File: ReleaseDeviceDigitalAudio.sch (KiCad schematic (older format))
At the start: 5 parts, among them J1 AudioJack3, J2 AudioJack3, J3 AudioJack3, J4 AudioJack3, J5 AudioJack3

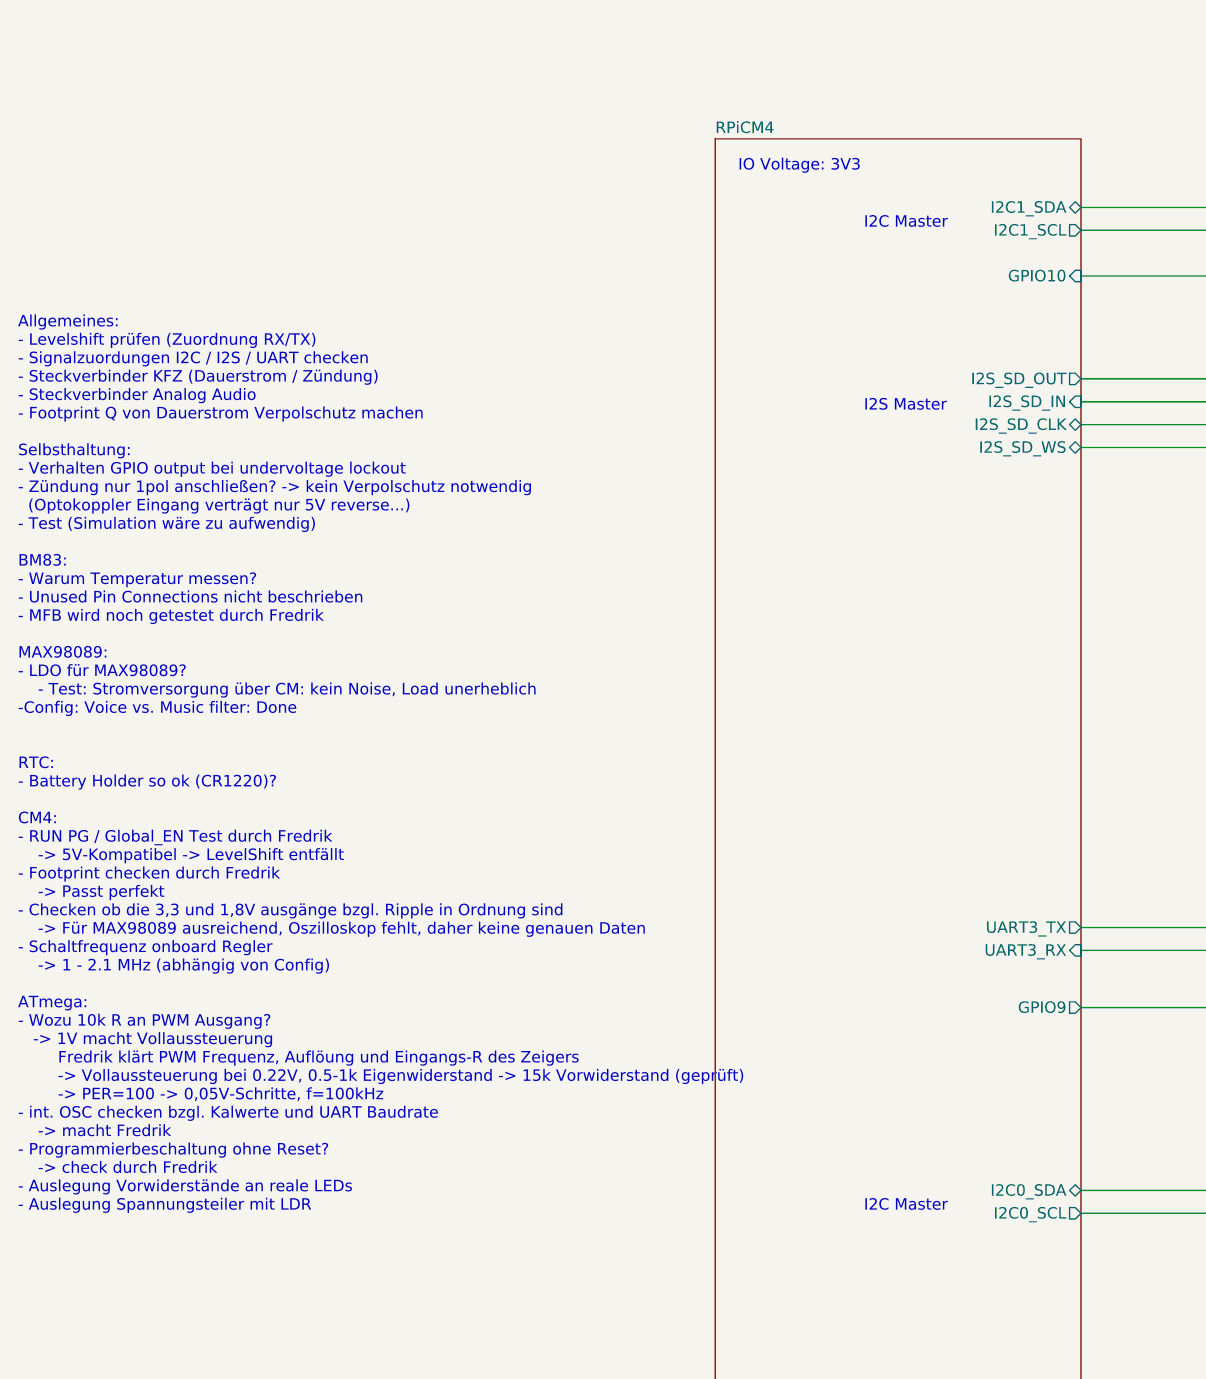
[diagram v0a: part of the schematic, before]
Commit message: - Kommentare aktualisiert
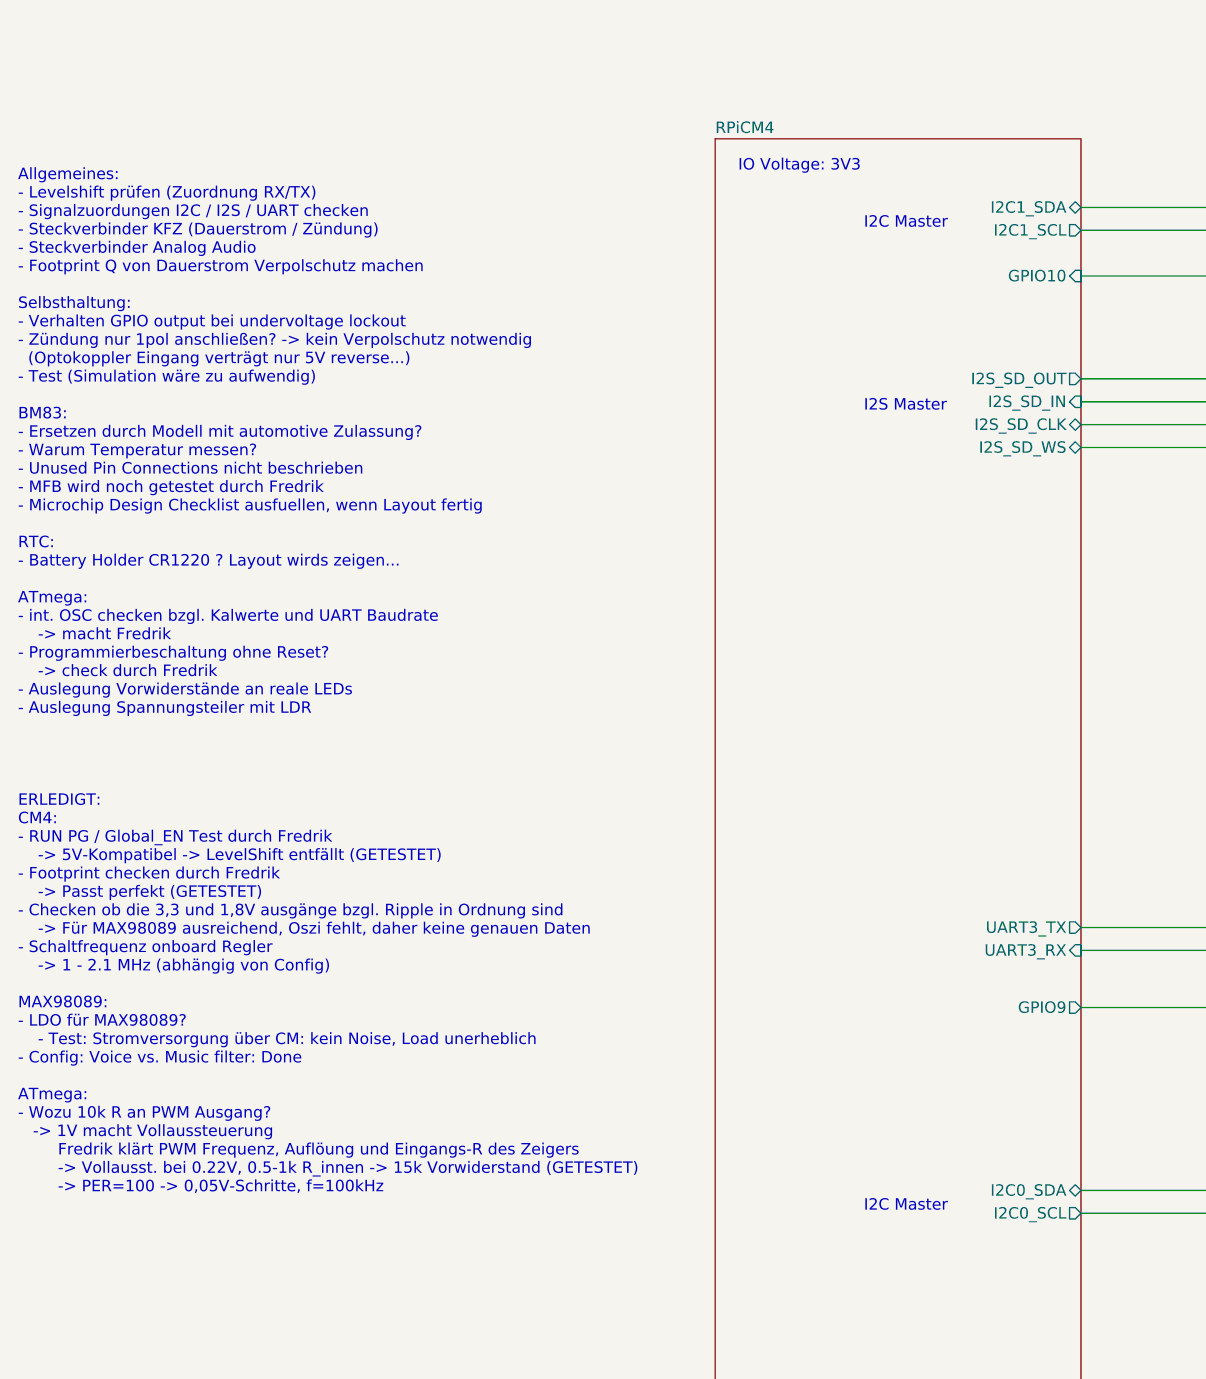
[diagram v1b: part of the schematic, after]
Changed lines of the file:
@@
 $EndComp
 Text Notes 900  5800 0    50   ~ 0
-Allgemeines: \n- Levelshift prüfen (Zuordnung RX/TX)\n- Signalzuordungen I2C / I2S / UART checken\n- Steckverbinder KFZ (Dauerstrom / Zündung)\n- Steckverbinder Analog Audio\n- Footprint Q von Dauerstrom Verpolschutz machen\n\nSelbsthaltung:\n- Verhalten GPIO output bei undervoltage lockout\n- Zündung nur 1pol anschließen? -> kein Verpolschutz notwendig\n  (Optokoppler Eingang verträgt nur 5V reverse...)\n- Test (Simulation wäre zu aufwendig)\n\nBM83:\n- Warum Temperatur messen?\n- Unused Pin Connections nicht beschrieben\n- MFB wird noch getestet durch Fredrik\n\nMAX98089:\n- LDO für MAX98089? \n    - Test: Stromversorgung über CM: kein Noise, Load unerheblich\n-Config: Voice vs. Music filter: Done\n\n\nRTC:\n- Battery Holder so ok (CR1220)?\n\nCM4: \n- RUN PG / Global_EN Test durch Fredrik\n    -> 5V-Kompatibel -> LevelShift entfällt\n- Footprint checken durch Fredrik\n    -> Passt perfekt\n- Checken ob die 3,3 und 1,8V ausgänge bzgl. Ripple in Ordnung sind\n    -> Für MAX98089 ausreichend, Oszilloskop fehlt, daher keine genauen Daten\n- Schaltfrequenz onboard Regler\n    -> 1 - 2.1 MHz (abhängig von Config)\n\nATmega:\n- Wozu 10k R an PWM Ausgang?\n   -> 1V macht Vollaussteuerung\n        Fredrik klärt PWM Frequenz, Auflöung und Eingangs-R des Zeigers\n        -> Vollaussteuerung bei 0.22V, 0.5-1k Eigenwiderstand -> 15k Vorwiderstand (geprüft)\n        -> PER=100 -> 0,05V-Schritte, f=100kHz\n- int. OSC checken bzgl. Kalwerte und UART Baudrate\n    -> macht Fredrik\n- Programmierbeschaltung ohne Reset?\n    -> check durch Fredrik\n- Auslegung Vorwiderstände an reale LEDs\n- Auslegung Spannungsteiler mit LDR\n
+Allgemeines: \n- Levelshift prüfen (Zuordnung RX/TX)\n- Signalzuordungen I2C / I2S / UART checken\n- Steckverbinder KFZ (Dauerstrom / Zündung)\n- Steckverbinder Analog Audio\n- Footprint Q von Dauerstrom Verpolschutz machen\n\nSelbsthaltung:\n- Verhalten GPIO output bei undervoltage lockout\n- Zündung nur 1pol anschließen? -> kein Verpolschutz notwendig\n  (Optokoppler Eingang verträgt nur 5V reverse...)\n- Test (Simulation wäre zu aufwendig)\n\nBM83:\n- Ersetzen durch Modell mit automotive Zulassung?\n- Warum Temperatur messen?\n- Unused Pin Connections nicht beschrieben\n- MFB wird noch getestet durch Fredrik\n- Microchip Design Checklist ausfuellen, wenn Layout fertig\n\nRTC:\n- Battery Holder CR1220 ? Layout wirds zeigen...\n\nATmega:\n- int. OSC checken bzgl. Kalwerte und UART Baudrate\n    -> macht Fredrik\n- Programmierbeschaltung ohne Reset?\n    -> check durch Fredrik\n- Auslegung Vorwiderstände an reale LEDs\n- Auslegung Spannungsteiler mit LDR\n\n\n\n\nERLEDIGT:\nCM4: \n- RUN PG / Global_EN Test durch Fredrik\n    -> 5V-Kompatibel -> LevelShift entfällt (GETESTET)\n- Footprint checken durch Fredrik\n    -> Passt perfekt (GETESTET)\n- Checken ob die 3,3 und 1,8V ausgänge bzgl. Ripple in Ordnung sind\n    -> Für MAX98089 ausreichend, Oszi fehlt, daher keine genauen Daten\n- Schaltfrequenz onboard Regler\n    -> 1 - 2.1 MHz (abhängig von Config)\n\nMAX98089:\n- LDO für MAX98089? \n    - Test: Stromversorgung über CM: kein Noise, Load unerheblich\n- Config: Voice vs. Music filter: Done\n\nATmega:\n- Wozu 10k R an PWM Ausgang?\n   -> 1V macht Vollaussteuerung\n        Fredrik klärt PWM Frequenz, Auflöung und Eingangs-R des Zeigers\n        -> Vollausst. bei 0.22V, 0.5-1k R_innen -> 15k Vorwiderstand (GETESTET)\n        -> PER=100 -> 0,05V-Schritte, f=100kHz\n\n
 Wire Wire Line
 	9650 2400 12850 2400
